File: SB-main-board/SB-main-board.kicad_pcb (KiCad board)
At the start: 4 copper layers, 53 x 40 mm, 94 parts, among them J1 XT30PB_IN, J2 USB_C_Receptacle_USB2.0_16P, J3 Excluder, J4 PT100, J5 Hotend, J6 FAN2, J7 LDC, J8 FS, J9 FAN, Q1 BUK9M8R5-40EX, SW1 BOOT, U1 RP2040, U10 TMP235A2, U11 LP5912-3.3DRV, U2 W25Q16JVUXIQ, U3 TJA1042TK-3, U4 TPS54302, U5 LP5912-3.3DRV, U6 TMC2208-LA, U7 OR, U8 ADXL343, U9 MAX31865xTP, Y1 12MHz

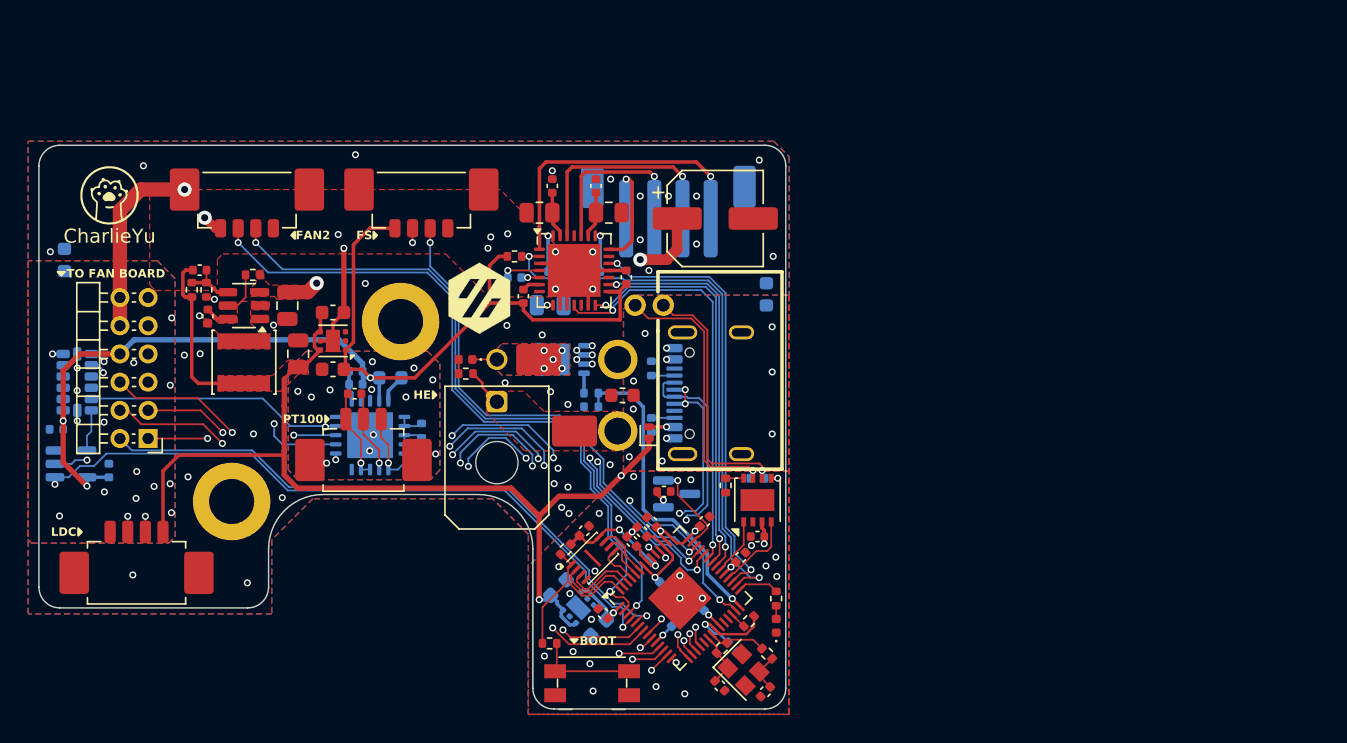
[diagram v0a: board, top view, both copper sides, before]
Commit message: fab: generate gerbers and bom
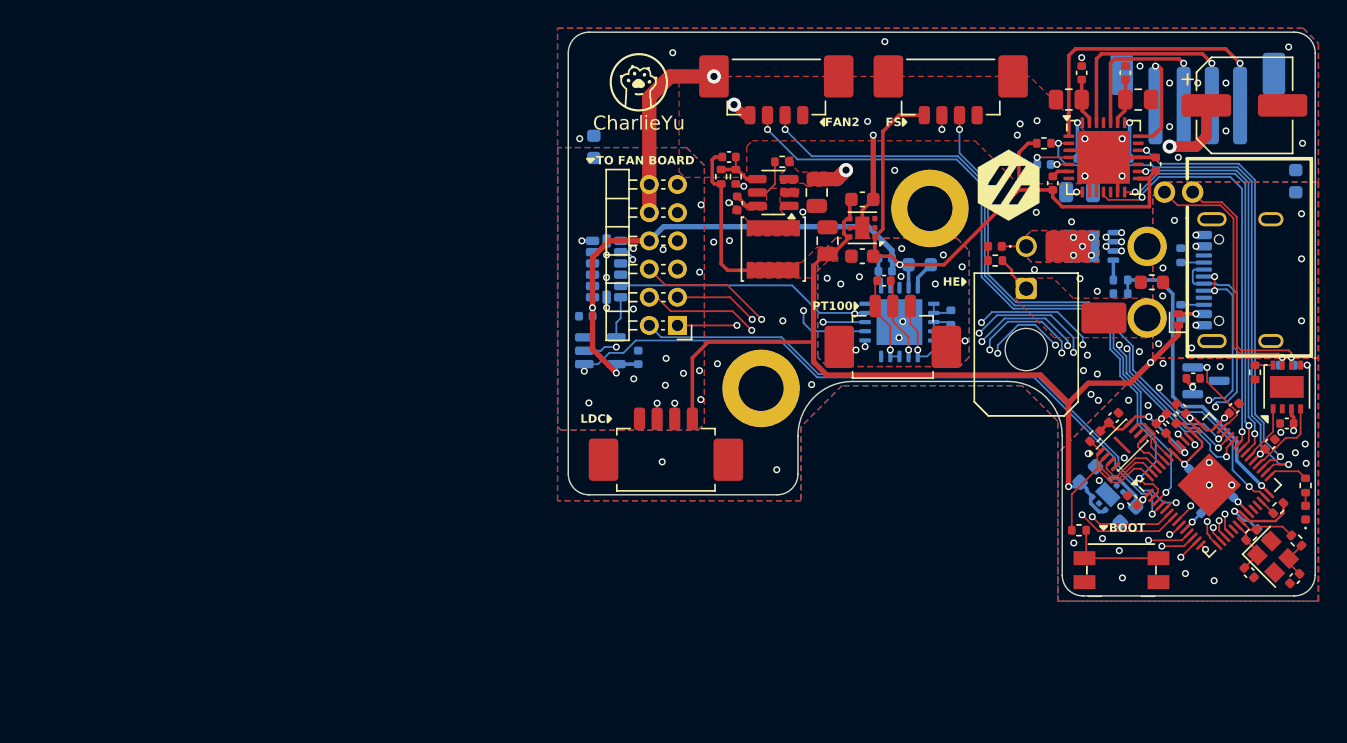
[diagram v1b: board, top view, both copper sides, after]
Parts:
- moved C10 38.4 mm to (167.0, 114.9)
- moved C13 38.4 mm to (160.7, 112.4)
- moved C21 38.4 mm to (158.9, 95.0)
- moved C28 38.4 mm to (153.6, 88.5)
- moved C3 38.4 mm to (168.7, 124.4)
- moved C30 38.4 mm to (122.1, 108.7)
- moved C6 38.4 mm to (160.0, 113.1)
- moved C8 38.4 mm to (166.4, 121.2)
- moved D1 38.4 mm to (169.5, 119.7)
- moved FB2 38.4 mm to (168.8, 96.2)
- moved H1 38.4 mm to (142.8, 98.1)
- moved J1 38.4 mm to (163.5, 101.6)
- moved J2 38.4 mm to (166.0, 103.2)
- moved J3 38.4 mm to (161.9, 90.3)
- moved R1 38.4 mm to (167.6, 119.4)
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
